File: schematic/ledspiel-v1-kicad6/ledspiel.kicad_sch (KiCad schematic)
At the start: 112 parts, among them J1 Conn_Battery, J3 USART Debug, J4 Micro_SD_Card, J5 USB_B_Micro, Q10 BSS138, Q11 BSS138, Q12 BSS138, Q13 BSS138, Q14 BSS138, Q40 IRLML6402, Q60 SFH300-3/4, U1 STM32F405RGTx, U2 USBLC6-2SC6, U3 MCP1640CH, U4 LP38693MP-3.3, U6 TSOP312xx, Y1 8MHz, Y2 32768Hz

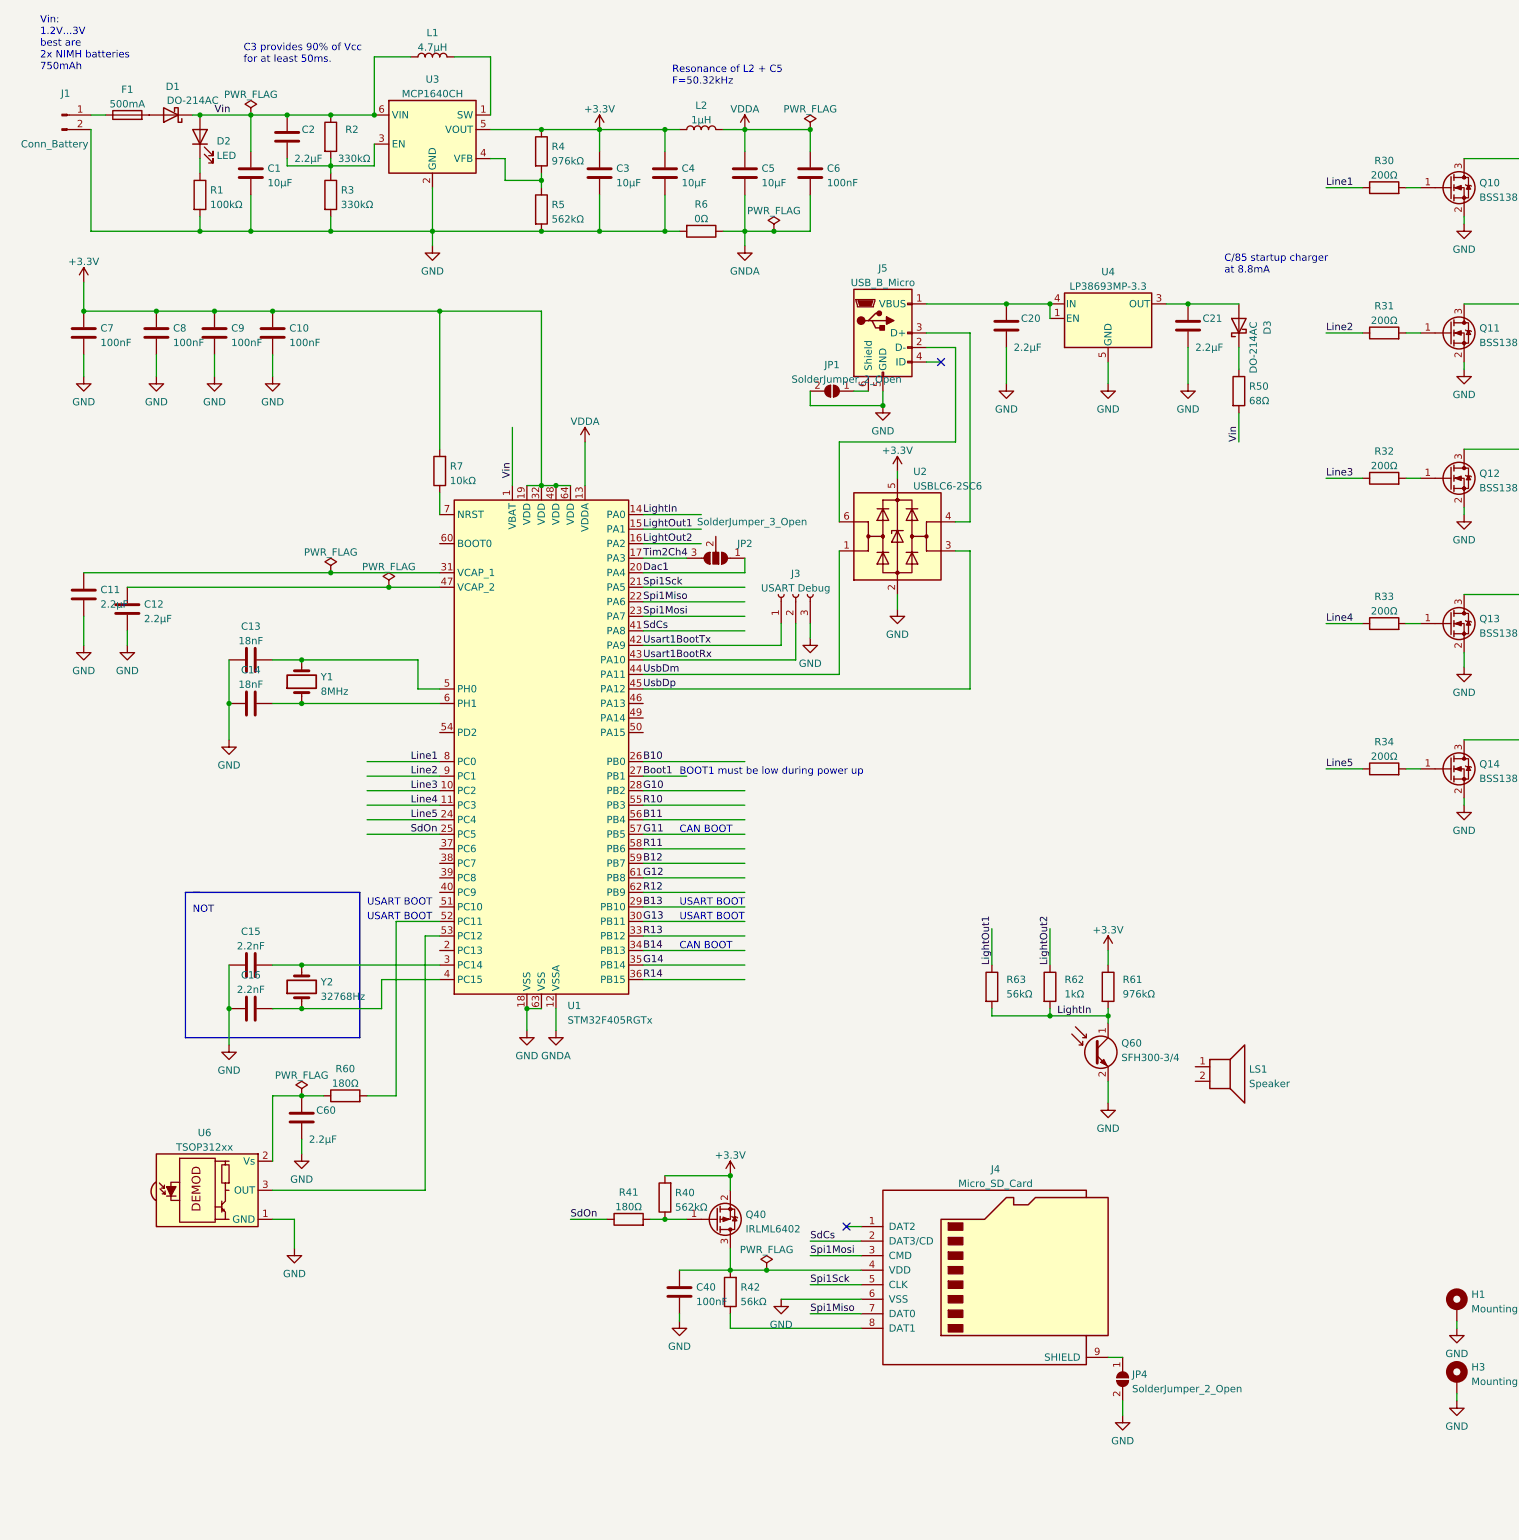
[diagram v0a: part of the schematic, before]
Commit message: WIP
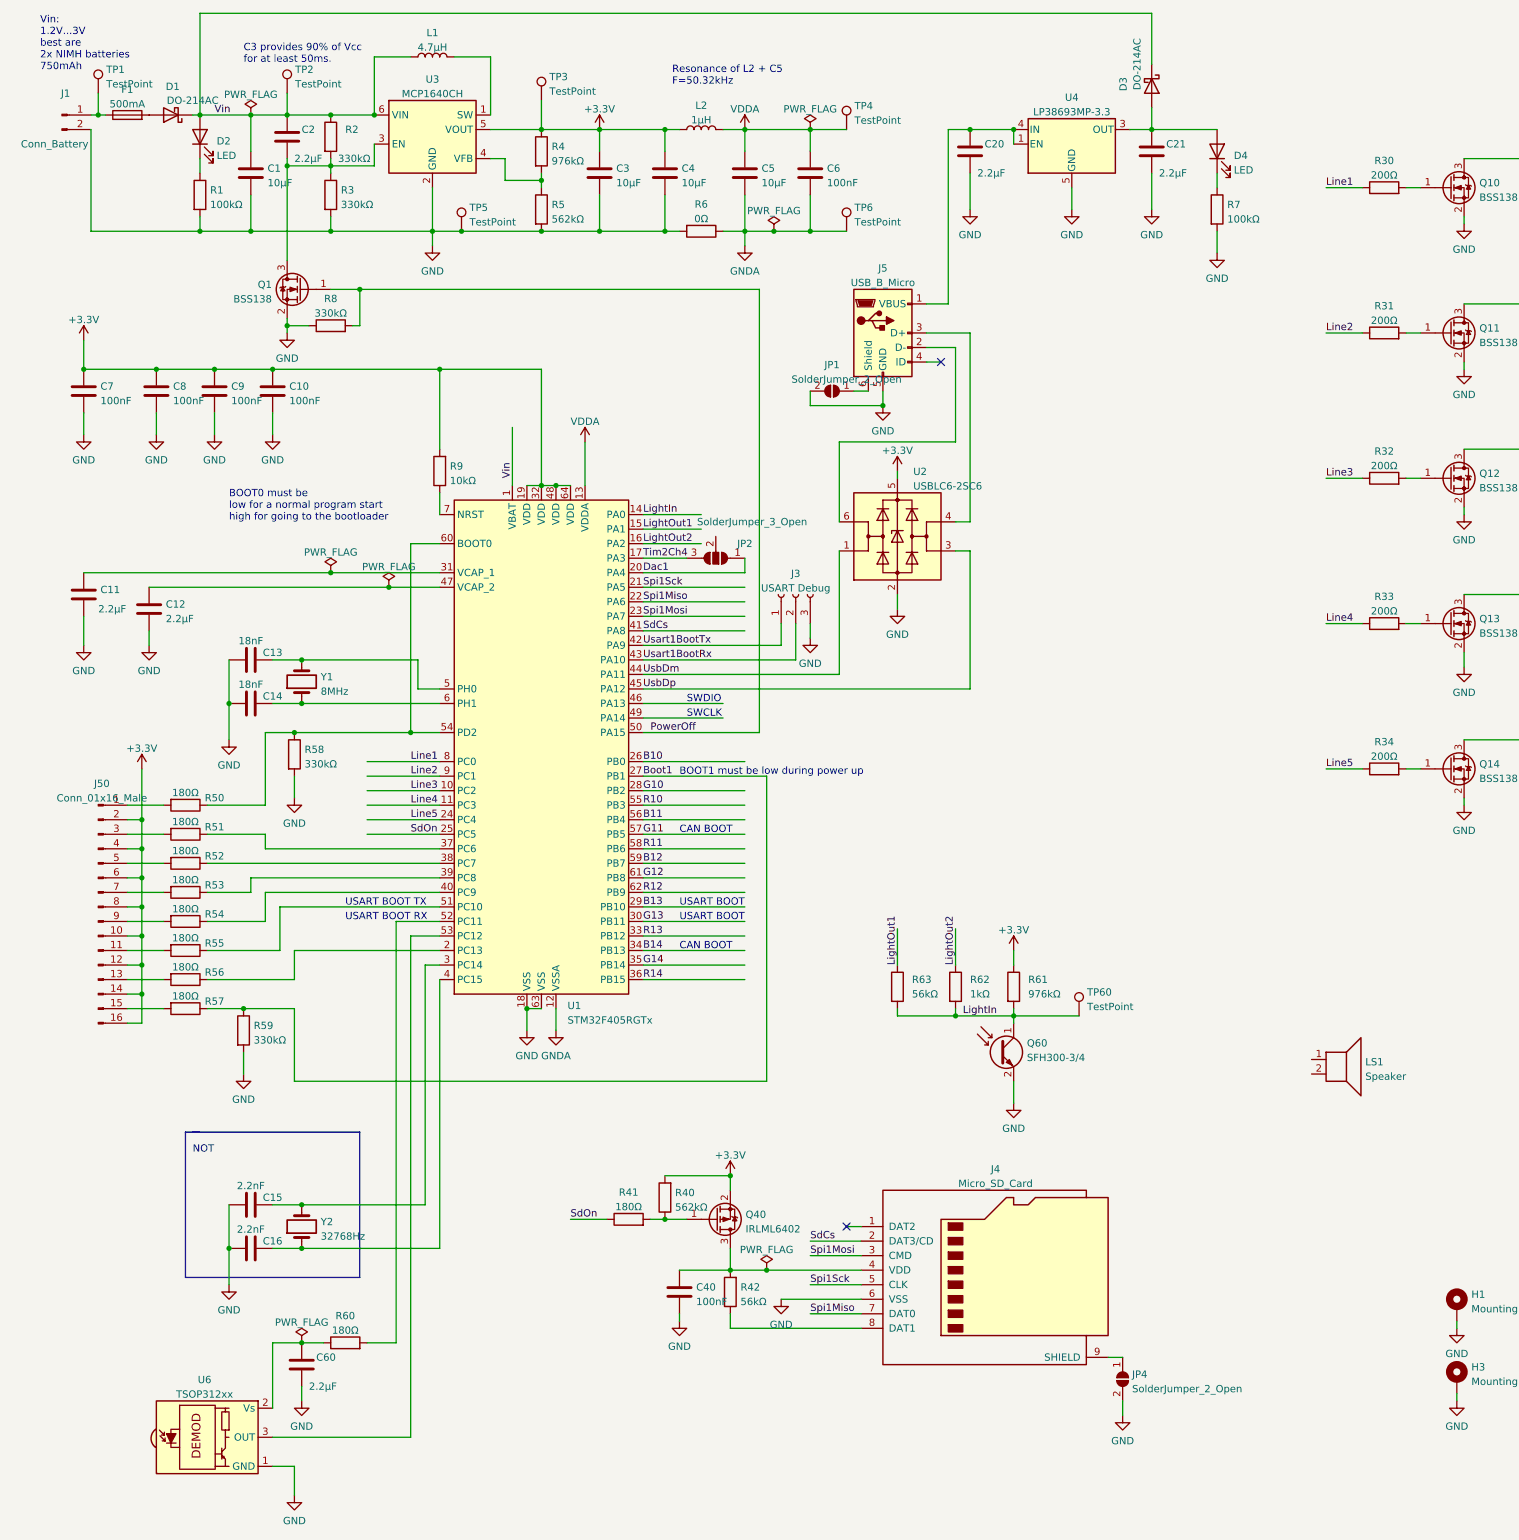
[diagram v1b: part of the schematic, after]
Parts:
- added D4: LED, symbol Device:LED
- added J50: Conn_01x16_Male, symbol Connector:Conn_01x16_Male
- added Q1: BSS138, Package_TO_SOT_SMD:SOT-23, symbol Transistor_FET:BSS138
- added R51, R52, R53, R54, R55, R56, R57: 180Ω, symbol Device:R
- added R58, R59, R8: 330kΩ, symbol Device:R
- added R7: 100kΩ, symbol Device:R
- added TP1, TP2, TP3, TP4, TP5, TP6, TP60: TestPoint, symbol Connector:TestPoint
- R50: value 68Ω -> 180Ω
- renumbered R7 to R9
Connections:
- net +3.3V: now also J50.10 (Pin_10), J50.12 (Pin_12), J50.14 (Pin_14), J50.16 (Pin_16), J50.2 (Pin_2), J50.4 (Pin_4), J50.6 (Pin_6), J50.8 (Pin_8), TP3.1
- net Boot1: now also R57.1, R59.1
- net GND: now also Q1.2 (S), R58.2, R59.2, R7.2, R8.1, TP5.1
- net GNDA: now also TP6.1
- net LightIn: now also TP60.1
- net VDDA: now also TP4.1
- net Vin: now also D3.1 (K), TP2.1; no longer R50.2
- net at C2.2, R2.2, R3.1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: now also Q1.3 (D)
- net at F1.1, J1.1 (Pin_1): now also TP1.1
- net at C21.1, D3.2 (A), U4.3 (OUT): now also D4.2 (A)
- net at R50.1: now also U1.54 (PD2), U1.60 (BOOT0), R58.1; no longer D3.1 (K)
- net at U1.2 (PC13): now also R56.1
- net at U1.37 (PC6): now also R51.1
- net at U1.38 (PC7): now also R52.1
- net at U1.39 (PC8): now also R53.1
- net at U1.40 (PC9): now also R54.1
- net PowerOff: now reaches U1.50 (PA15)
- net PowerOff: now also Q1.1 (G), R8.2
- net at U1.51 (PC10): now also R55.1
- new net: J50.1 (Pin_1), R50.2
- new net: J50.11 (Pin_11), R55.2
- new net: J50.13 (Pin_13), R56.2
- new net: J50.15 (Pin_15), R57.2
- new net: J50.3 (Pin_3), R51.2
- new net: J50.5 (Pin_5), R52.2
- new net: J50.7 (Pin_7), R53.2
- new net: J50.9 (Pin_9), R54.2
- new net: D4.1 (K), R7.1
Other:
- note added: "BOOT0 must be low for a normal program start high for going to the bootloader"
- note added: "SWCLK"
- note added: "SWDIO"
- note added: "USART BOOT RX"
- note added: "USART BOOT TX"
- note removed: "C/85 startup charger at 8.8mA"
- moved on the sheet: C10, C12, C15, C16, C20, C21, C60, C7, C8, C9, D3, LS1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
